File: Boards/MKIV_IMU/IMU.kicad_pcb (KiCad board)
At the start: 2 copper layers, 50.8 x 55.9 mm, 42 parts, among them J1 UF_4_VT, J4 CONN_02X03, U1 CAN_Transceiver, U2 TPS561201, U3 LM3480, U4 BMI088, U5 ATMEGA16M1, Y1 Crystal_SMD

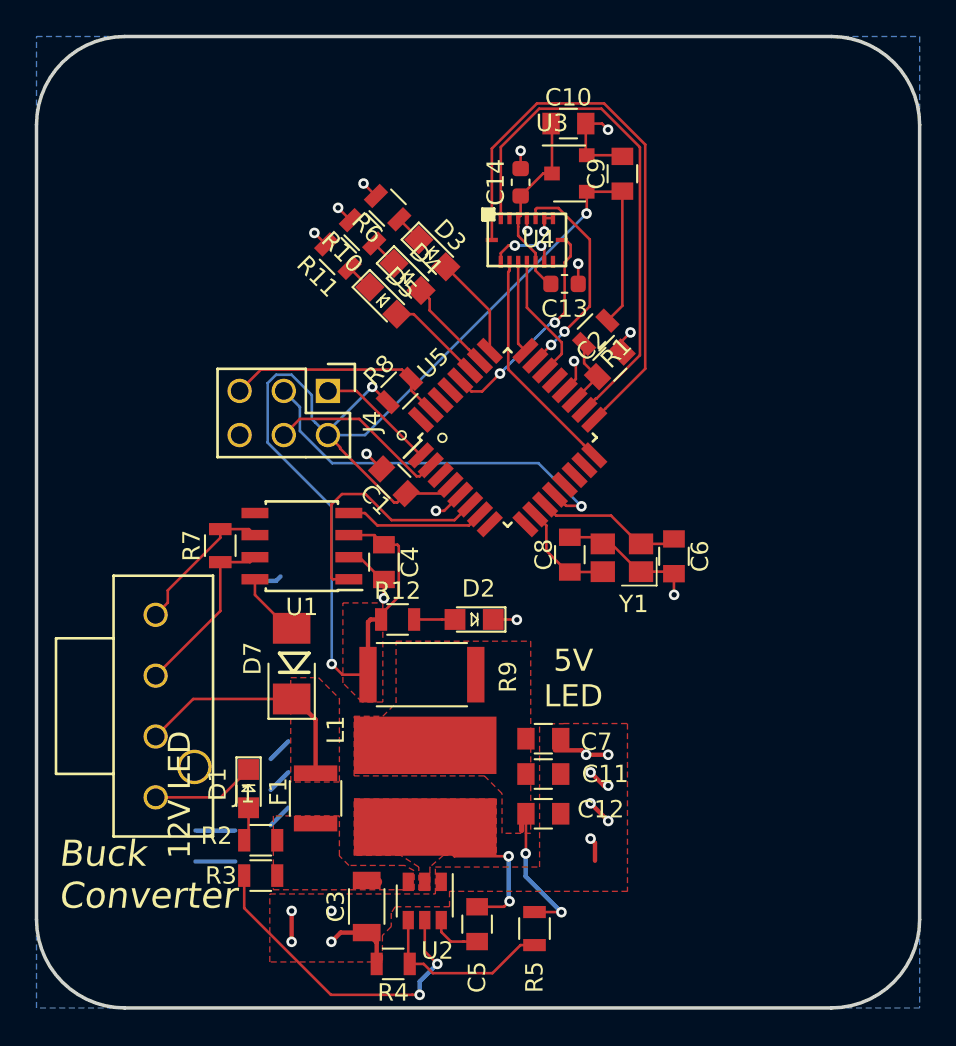
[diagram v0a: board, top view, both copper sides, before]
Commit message: even more layout changesgit add IMU.kicad_pcb-bak
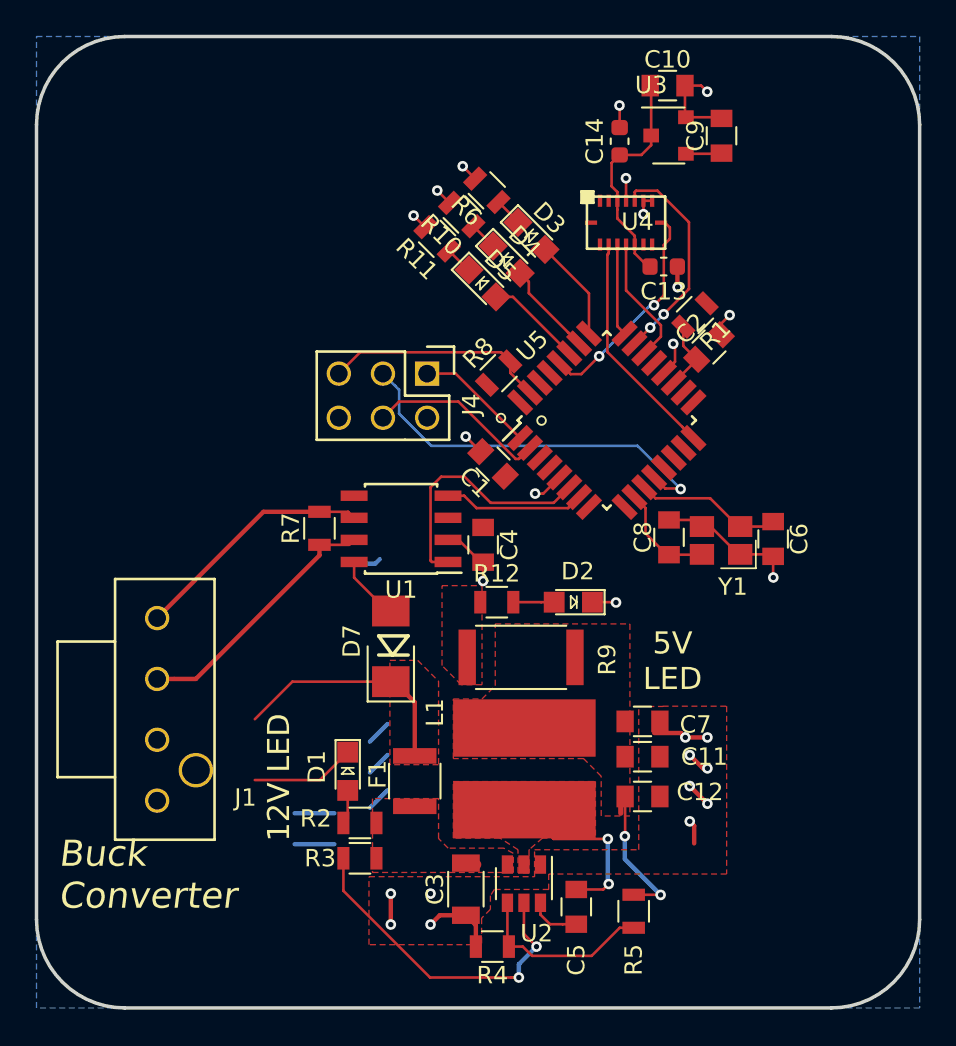
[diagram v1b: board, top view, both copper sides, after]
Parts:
- moved C14 6.17 mm to (149.1, 77.1)
- moved C10 6.11 mm to (151.9, 73.9)
- moved U3 6.11 mm to (150.9, 76.8)
- moved C9 6.11 mm to (155.0, 76.8)
- moved C11 5.79 mm to (150.4, 112.5)
- moved C12 5.79 mm to (150.4, 114.8)
- moved C6 5.79 mm to (157.9, 100.0)
- moved C7 5.79 mm to (150.4, 110.5)
- moved D5 5.79 mm to (141.2, 85.3)
- moved R10 5.79 mm to (140.0, 81.4)
- moved R12 5.79 mm to (142.0, 103.7)
- moved R2 5.79 mm to (134.2, 116.4)
- moved U5 5.79 mm to (148.4, 93.2)
- moved C1 5.79 mm to (141.8, 95.7)
- moved C5 5.79 mm to (146.6, 121.2)
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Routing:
- net VCC: track 83.0 -> 2.06 mm, vias 3 -> 0
- net /INT1: track 33.2 -> 0.00 mm
- net /INT2: track 30.4 -> 0.00 mm
- net /CANL: track 8.61 -> 14.0 mm
- net /CANH: track 10.2 -> 15.0 mm
- net /MISO2: track 4.02 -> 0.00 mm, vias 2 -> 0
- net /3.3V: track 11.2 -> 13.1 mm
- net GND: track 65.9 -> 66.7 mm
